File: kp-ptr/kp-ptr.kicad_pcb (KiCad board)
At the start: 4 copper layers, 31.6 x 101.5 mm, 174 parts, among them IC1 E22-900M22S, J1 ESP32_PROG_CON, J10 Conn_01x02, J11 Conn_01x02, J12 Conn_01x02, J13 Conn_01x02, J2 Conn_01x02, J3 Conn_01x02, J4 USB_C_Receptacle_USB2.0, J5 u.fl, J6 Conn_01x06_Male, J7 Conn_01x10_Male, J8 Conn_01x06_Male, J9 Conn_01x02_Male, Q1 NMOS_SOT23, Q2 DMC2025UFDB_v2, Q3 DMC2025UFDB_v2, Q4 DMC2025UFDB_v2, Q5 DMC2025UFDB_v2, U1 ESP32-S3FN8, U10 USBLC6-2SC6, U11 W25Q128JVS, U12 NL27WZU04DBVT1G, U2 MS560702BA03-50, U3 MMC5983MA, U4 H3LIS331, U5 L76-L, U6 NJG1156PCD, U7 LSM6DSO32, U8 AZ1117CH-5.0TRG1, U9 LDFM33PVR, Y1 7M40000005-40MHz

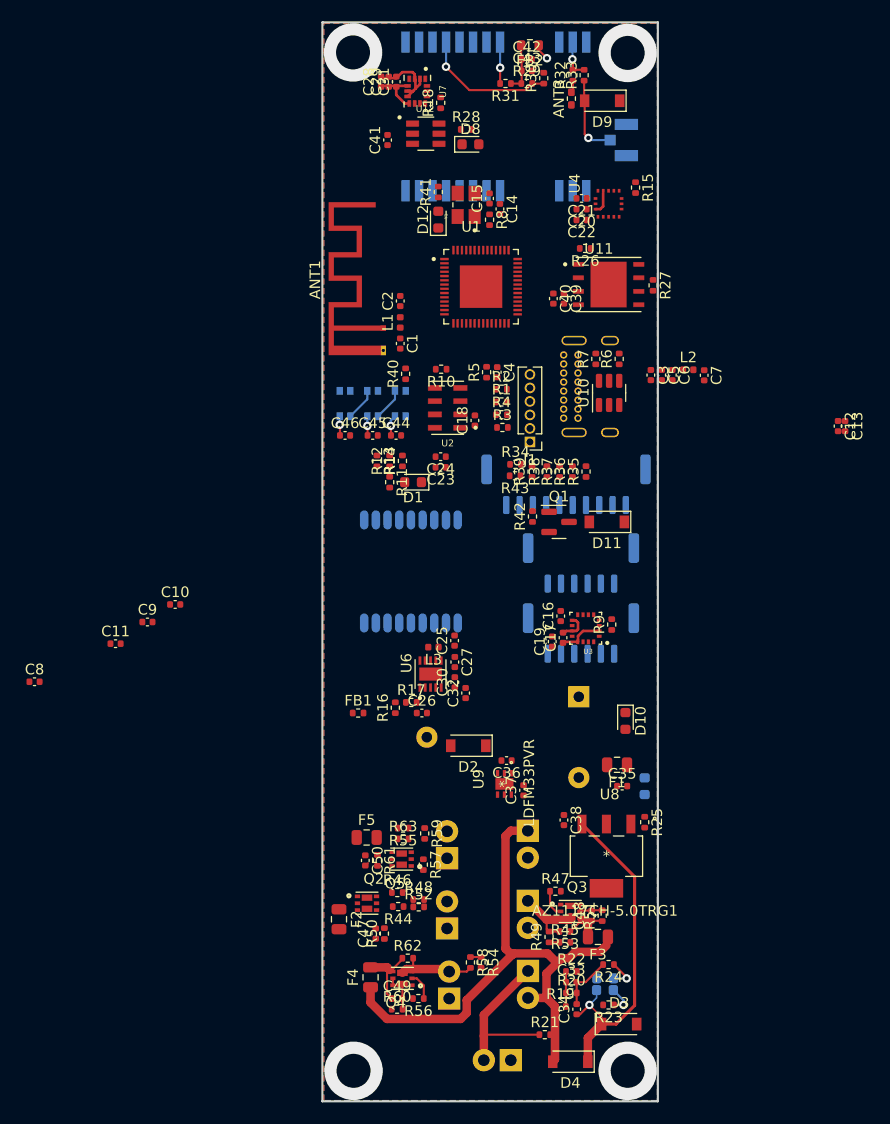
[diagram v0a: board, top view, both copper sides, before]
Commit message: PCB update
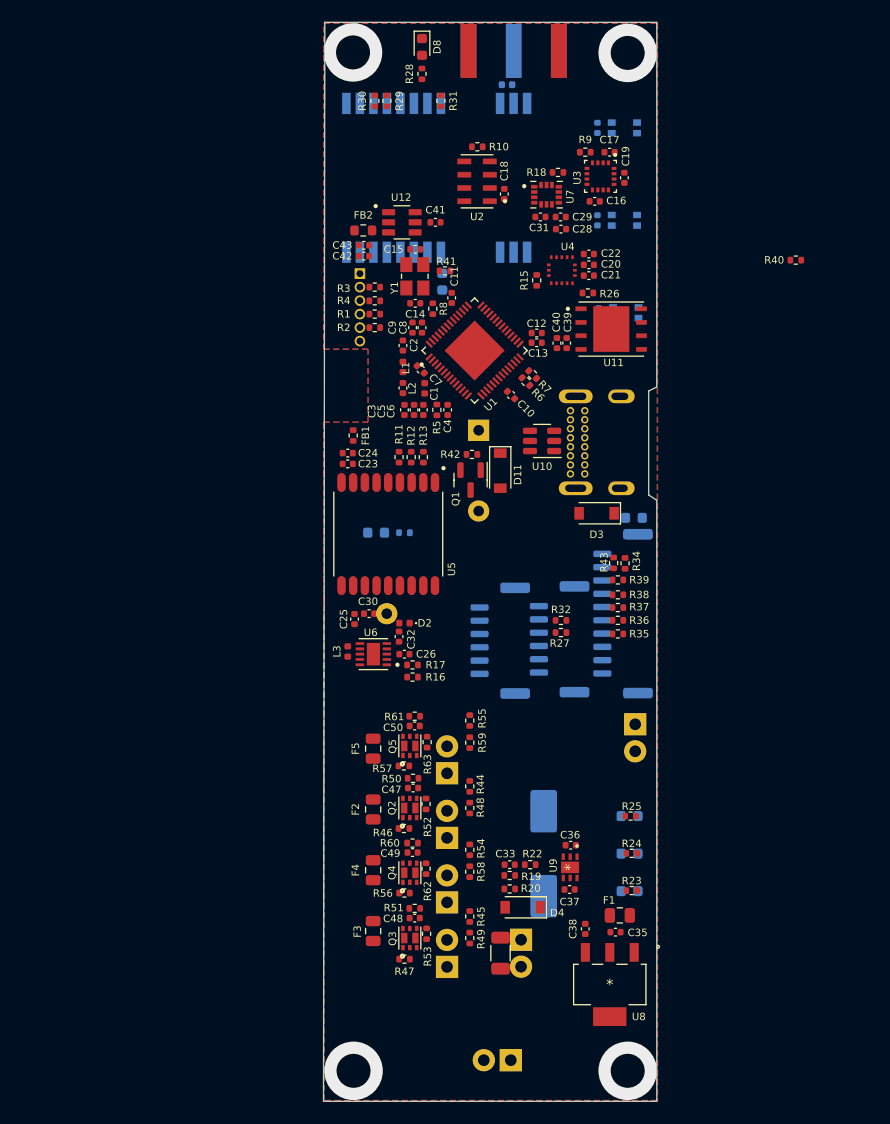
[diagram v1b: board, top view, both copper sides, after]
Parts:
- removed ANT1: PCB_antenna, RF_Antenna:Texas_SWRA117D_2.4GHz_Right
- removed ANT3: TBD, Resistor_SMD:R_0402_1005Metric_Pad0.72x0.64mm_HandSolder
- removed C27: DNP, Capacitor_SMD:C_0402_1005Metric
- removed R33: 0R, Resistor_SMD:R_0402_1005Metric
- C34: footprint Capacitor_SMD:C_0402_1005Metric -> Capacitor_SMD:CP_Elec_10x10; moved to B.Cu
- C44, C45, C46, D1, D10, D12, J1, R14: moved to B.Cu
- D2: footprint Diode_SMD:D_SOD-123 -> Diode_SMD:D_0402_1005Metric
- D9: footprint Diode_SMD:D_SOD-123 -> Diode_SMD:D_0402_1005Metric; moved to B.Cu
- J4: footprint Connector_USB:USB_C_Receptacle_GCT_USB4085 -> KP-PTR_lib:USB_C_213716
- J5: footprint Connector_Coaxial:U.FL_Hirose_U.FL-R-SMT-1_Vertical -> Connector_Coaxial:SMA_Amphenol_132289_EdgeMount
- R21: footprint Resistor_SMD:R_0402_1005Metric -> Resistor_SMD:R_1206_3216Metric
- R27: value 100k -> 10k
- R32: value DNP -> 10k
- U5: moved to F.Cu
- moved R32 51.3 mm to (163.3, 88.0), turned to 0 degrees
- moved C8 49.4 mm to (150.2, 60.5), turned to 90 degrees
- moved D3 48.1 mm to (166.7, 77.9), turned to 180 degrees
- moved C17 45.9 mm to (167.9, 43.9), turned to 0 degrees
- moved C11 45.4 mm to (153.0, 57.7), turned to 90 degrees
- moved R9 44.5 mm to (165.6, 43.9), turned to 0 degrees
- moved C19 44.2 mm to (169.3, 46.4)
- moved U3 42.6 mm to (167.0, 46.2), turned to -90 degrees
- moved C16 39.2 mm to (166.5, 48.6), turned to 180 degrees
- moved R40 38.2 mm to (185.4, 54.1), turned to 180 degrees
- moved C46 37.4 mm to (166.8, 41.7), turned to -90 degrees
- moved C9 37.3 mm to (149.4, 60.5), turned to 90 degrees
- moved C10 37.3 mm to (158.6, 66.8), turned to -45 degrees
- moved D15 36.9 mm to (169.3, 41.7), turned to 180 degrees
- moved R27 33.8 mm to (163.3, 89.2), turned to 0 degrees
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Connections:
- C30 pad 1: Net-(C30-Pad1) -> Net-(ANT2-Pad1)
- C30 pad 2: Net-(C27-Pad2) -> Net-(C25-Pad2)
- C32 pad 2: Net-(C30-Pad1) -> Net-(C32-Pad2)
- C38 pad 1: VDD -> VCC
- D8 pad 1: Net-(D8-Pad1) -> Net-(U12-Pad6)
- D9 pad 2: Net-(D9-Pad2) -> Net-(IC1-Pad21)
- J10 pad 1: Net-(J10-Pad1) -> Earth
- J10 pad 2: Earth -> Net-(J10-Pad2)
- J11 pad 1: Net-(J11-Pad1) -> Earth
- J11 pad 2: Earth -> Net-(J11-Pad2)
- J13 pad 1: Net-(J13-Pad1) -> Earth
- J13 pad 2: Earth -> Net-(J13-Pad2)
- J3 pad 1: +BATT -> VCC
- J3 pad 2: VCC -> +BATT
- J5 pad 1: Net-(D9-Pad2) -> Net-(IC1-Pad21)
- Q2 pad 3: Net-(J10-Pad1) -> Net-(J10-Pad2)
- Q3 pad 3: Net-(J11-Pad1) -> Net-(J11-Pad2)
- Q5 pad 3: Net-(J13-Pad1) -> Net-(J13-Pad2)
- R27 pad 1: +3V3 -> I2C_SCL
- R27 pad 2: SPI_CLK -> +3V3
- R32 pad 1: Net-(ANT3-Pad2) -> I2C_SDA
- R32 pad 2: Net-(IC1-Pad21) -> +3V3
- R48 pad 2: Net-(J10-Pad1) -> Net-(J10-Pad2)
- R49 pad 2: Net-(J11-Pad1) -> Net-(J11-Pad2)
- R52 pad 2: Net-(J10-Pad1) -> Net-(J10-Pad2)
- R53 pad 2: Net-(J11-Pad1) -> Net-(J11-Pad2)
- R59 pad 2: Net-(J13-Pad1) -> Net-(J13-Pad2)
- R63 pad 2: Net-(J13-Pad1) -> Net-(J13-Pad2)
- U10 pad 1: Net-(J4-PadA6) -> Net-(J4-PadA7)
- U10 pad 3: Net-(J4-PadA7) -> Net-(J4-PadA6)
- U10 pad 4: USB_DM -> USB_DP
- U10 pad 6: USB_DP -> USB_DM
- U12 pad 4: Net-(D8-Pad1) -> Net-(IC1-Pad6)
- U12 pad 6: Net-(IC1-Pad6) -> Net-(U12-Pad6)
- U6 pad 5: Net-(C30-Pad1) -> Net-(C32-Pad2)
- U8 pad 3: VDD -> VCC
- U8 pad 4: unconnected-(U8-Pad4) -> Net-(C35-Pad1)
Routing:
- net VCC: track 54.2 -> 0.00 mm
- net VDD: track 32.5 -> 0.00 mm, vias 1 -> 0
- net Earth: track 18.0 -> 0.02 mm
- net +3V3: track 16.4 -> 0.00 mm, vias 4 -> 0
- net +BATT: track 15.4 -> 0.00 mm
- net RF_RST: track 12.7 -> 0.00 mm, vias 1 -> 0
- net Net-(J12-Pad2): track 7.82 -> 0.00 mm
- net Net-(D9-Pad2): track 7.69 -> 0.00 mm, vias 1 -> 0
- net Net-(J11-Pad1): track 7.15 -> 0.00 mm
- net Net-(C49-Pad1): track 6.60 -> 0.00 mm
- net +3.3VP: track 4.61 -> 0.00 mm
- net Net-(C48-Pad1): track 4.51 -> 0.00 mm
- net Net-(C49-Pad2): track 3.98 -> 0.00 mm
- net SPI_CS_LORA: track 3.92 -> 0.00 mm, vias 1 -> 0
- net Net-(C48-Pad2): track 3.75 -> 0.00 mm
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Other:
- board size 31.6 x 101.5 mm -> 31.4 x 101.5 mm
